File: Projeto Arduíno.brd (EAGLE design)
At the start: 180.3 x 64.9 mm, 18 parts, among them U1 ARDUINO-UNO-R3-SHIELD

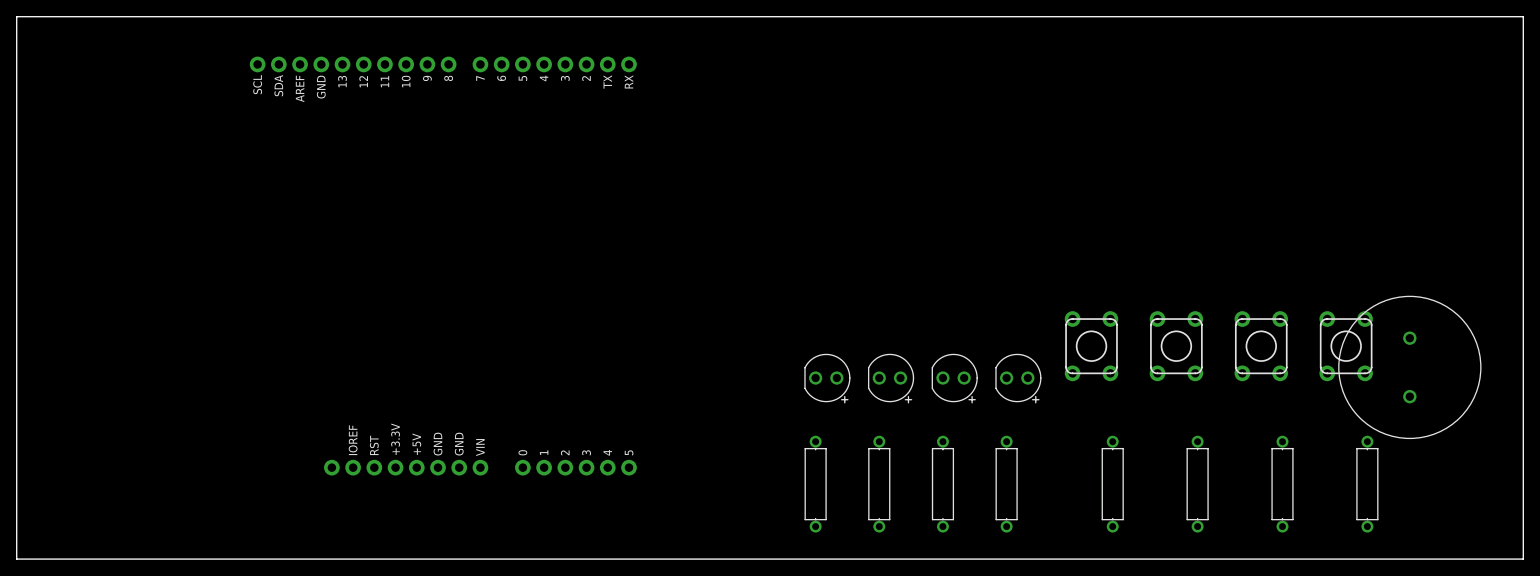
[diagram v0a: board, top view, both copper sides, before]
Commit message: Add files via upload
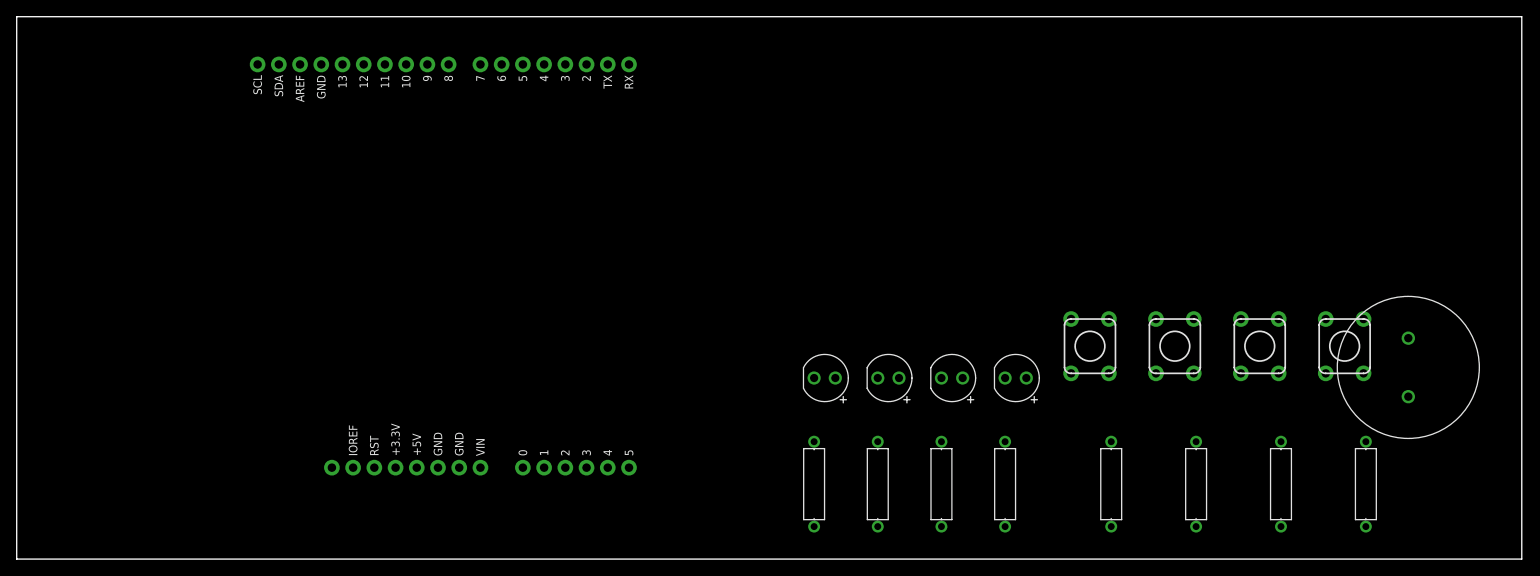
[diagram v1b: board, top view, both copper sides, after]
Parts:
- moved D1 0.18 mm to (96.7, 21.7)
- moved PIEZO1 0.18 mm to (166.6, 22.9)
- moved R5 0.18 mm to (131.0, 8.97)
- moved R6 0.18 mm to (141.2, 8.97)
- moved R7 0.18 mm to (151.3, 8.97)
- moved R8 0.18 mm to (161.5, 8.97)
- moved S3 0.18 mm to (148.8, 25.5)
- moved S4 0.18 mm to (158.9, 25.5)
- moved D2 0.18 mm to (104.3, 21.7)
- moved D3 0.18 mm to (112.0, 21.7)
- moved D4 0.18 mm to (119.6, 21.7)
- moved R1 0.18 mm to (95.4, 8.97)
- moved R2 0.18 mm to (103.1, 8.97)
- moved R3 0.18 mm to (110.7, 8.97)
- moved R4 0.18 mm to (118.3, 8.97)
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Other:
- board size 180.3 x 64.9 mm -> 180.1 x 64.9 mm
